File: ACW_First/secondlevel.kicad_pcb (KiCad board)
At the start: 2 copper layers, 103 x 65 mm, 70 parts, among them J11 24VDC, J12 Conn_01x02_Pin, J13 Conn_01x04_Socket, J14 Conn_01x02_Pin, J2 Conn_01x03_Pin, J3 3.8VDC, J4 5VDC, J5 12VDC, U1 MP1584EN, U2 MP1584EN, U3 MP1584EN

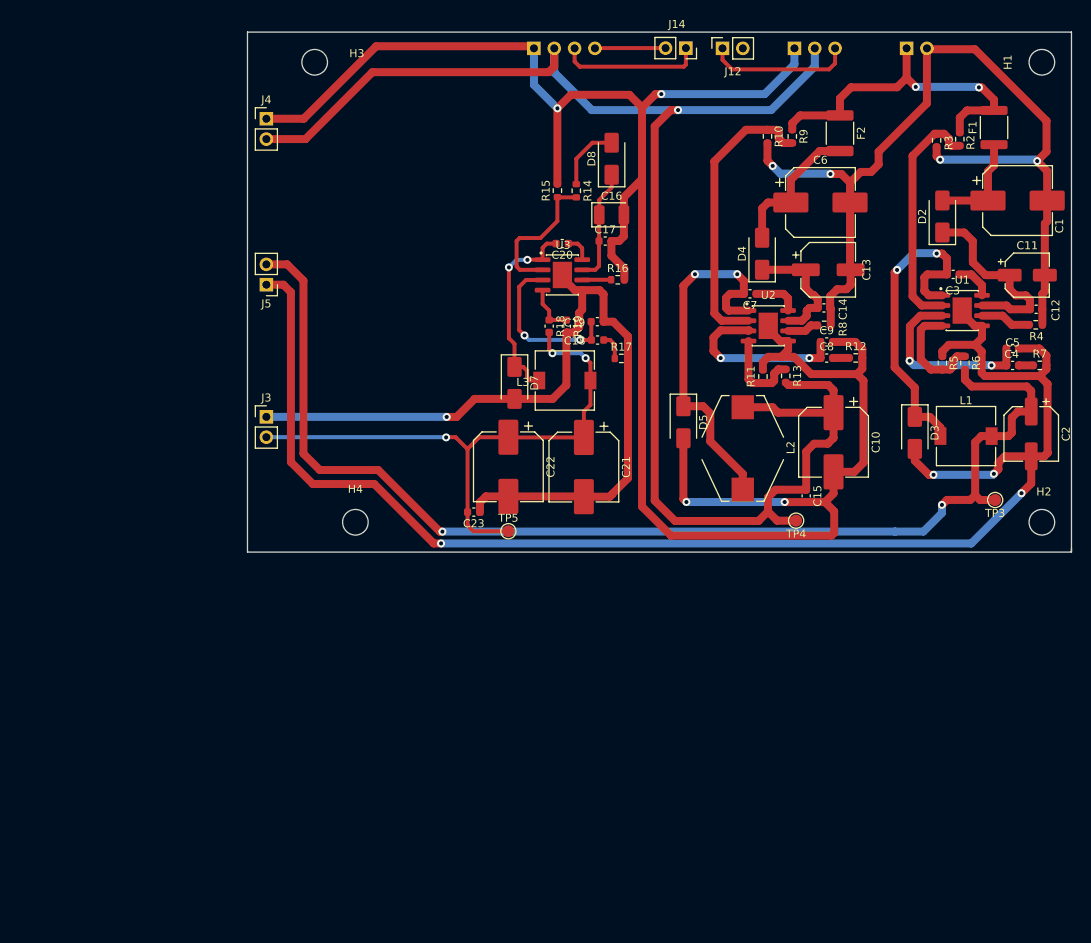
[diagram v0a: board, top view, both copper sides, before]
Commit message: okok
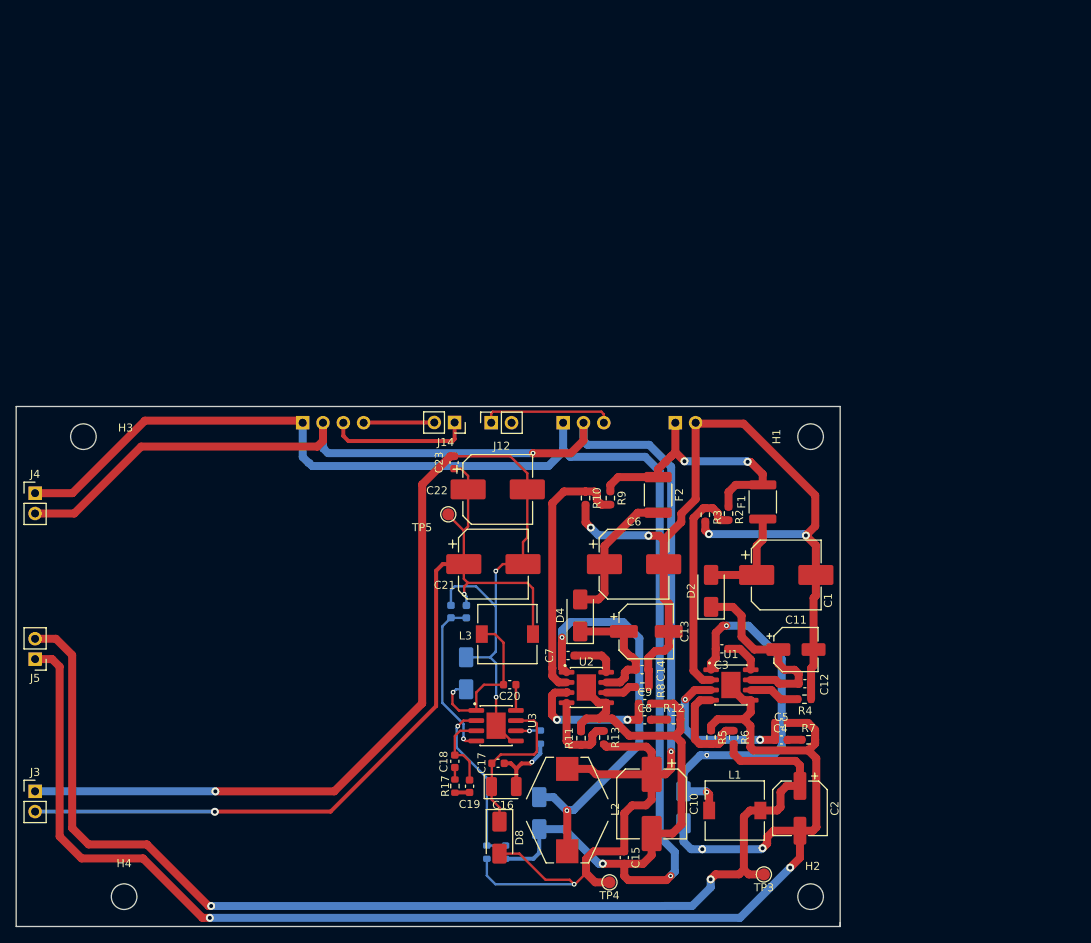
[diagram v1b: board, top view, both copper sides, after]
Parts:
- D3, D5, D7, R14, R15, R16, R18, R19: moved to B.Cu
- moved D8 86.0 mm to (558.2, 205.3), turned to -90 degrees
- moved R14 83.4 mm to (556.6, 207.1), turned to 90 degrees
- moved R15 82.9 mm to (559.0, 207.1), turned to -90 degrees
- moved C16 72.7 mm to (558.8, 198.9)
- moved C17 66.6 mm to (558.0, 196.0)
- moved C19 60.2 mm to (554.5, 198.9), turned to -90 degrees
- moved R16 58.0 mm to (563.3, 192.7), turned to -90 degrees
- moved R17 57.4 mm to (552.7, 198.8), turned to -90 degrees
- moved U3 57.0 mm to (557.8, 191.3)
- moved C18 55.6 mm to (552.6, 195.8), turned to -90 degrees
- moved C20 55.5 mm to (559.5, 186.2)
- moved C11 55.0 mm to (595.3, 181.8)
- moved C12 55.0 mm to (596.4, 186.1)
- moved C3 55.0 mm to (586.0, 181.7)
- moved U1 55.0 mm to (587.2, 186.2)
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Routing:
- net /5VDC to 3.8VDC/3.8VDC: track 73.6 -> 112.4 mm, vias 3 -> 2
- net Net-(U3-FB): track 6.22 -> 20.3 mm, vias 0 -> 1
- net /5VDC to 3.8VDC/COMP INPUT: track 20.5 -> 9.84 mm, vias 2 -> 0
- net GND: track 664.9 -> 674.8 mm, vias 13 -> 14
- net /24VDC: track 42.2 -> 34.7 mm
- net Net-(D3-K): track 40.9 -> 47.5 mm, vias 2 -> 3
- net Net-(D8-K): track 14.4 -> 20.2 mm
- net /24VDC to 5VDC/COMP INPUT: track 22.4 -> 17.6 mm
- net Net-(D5-K): track 46.8 -> 51.4 mm
- net Net-(D7-K): track 25.0 -> 21.1 mm, vias 2 -> 1
- net /24VDC to 5VDC/1.65V: track 36.2 -> 32.7 mm
- net /5VDC to 3.8VDC/1.65V: track 18.1 -> 21.5 mm, vias 0 -> 1
- net /5VDC: track 202.8 -> 205.1 mm, vias 1 -> 3
- net /24VDC to 12VDC/1.65V: track 29.8 -> 27.6 mm
- net /24VDC to 12VDC/COMP INPUT: track 23.4 -> 21.4 mm
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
